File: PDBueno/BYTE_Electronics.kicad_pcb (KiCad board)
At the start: 2 copper layers, 99 x 42 mm, 3 parts, among them J9 Screw_Terminal_01x02, U1 LM2596S-3.3

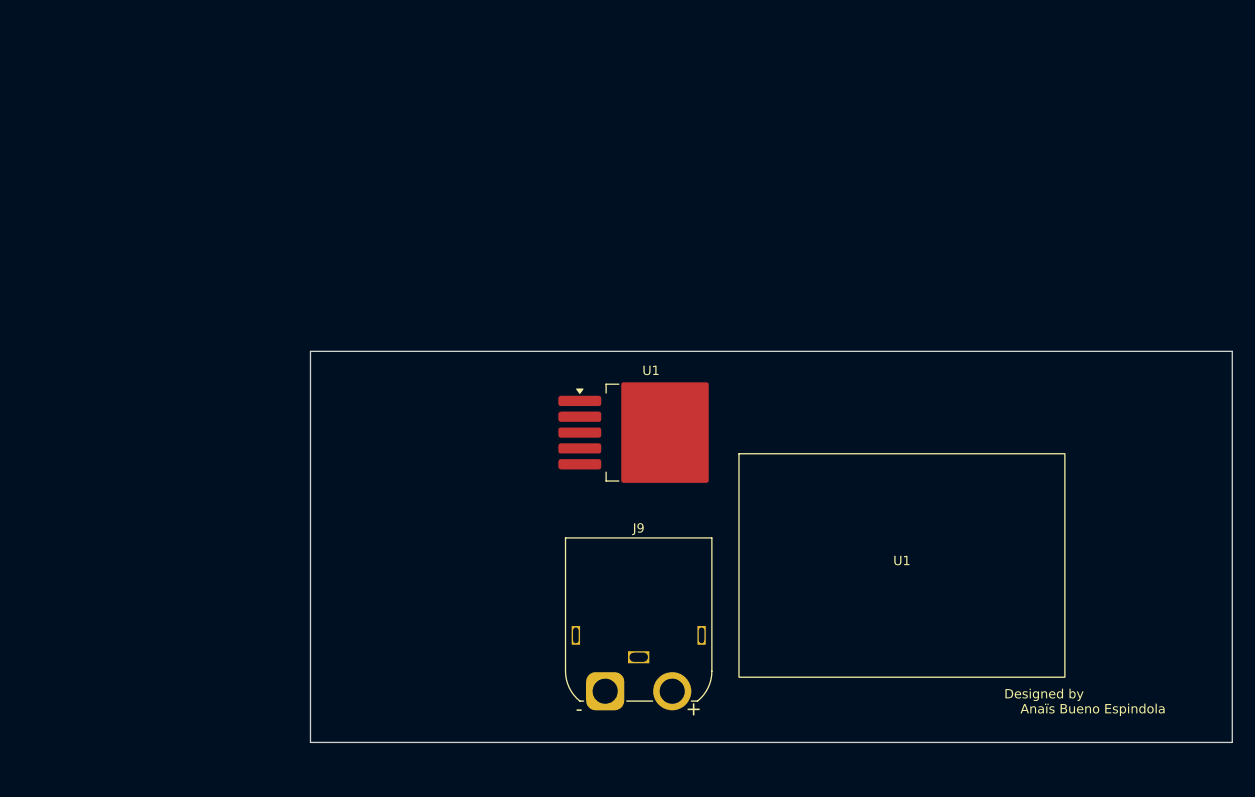
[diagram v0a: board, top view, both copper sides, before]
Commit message: PCB routing
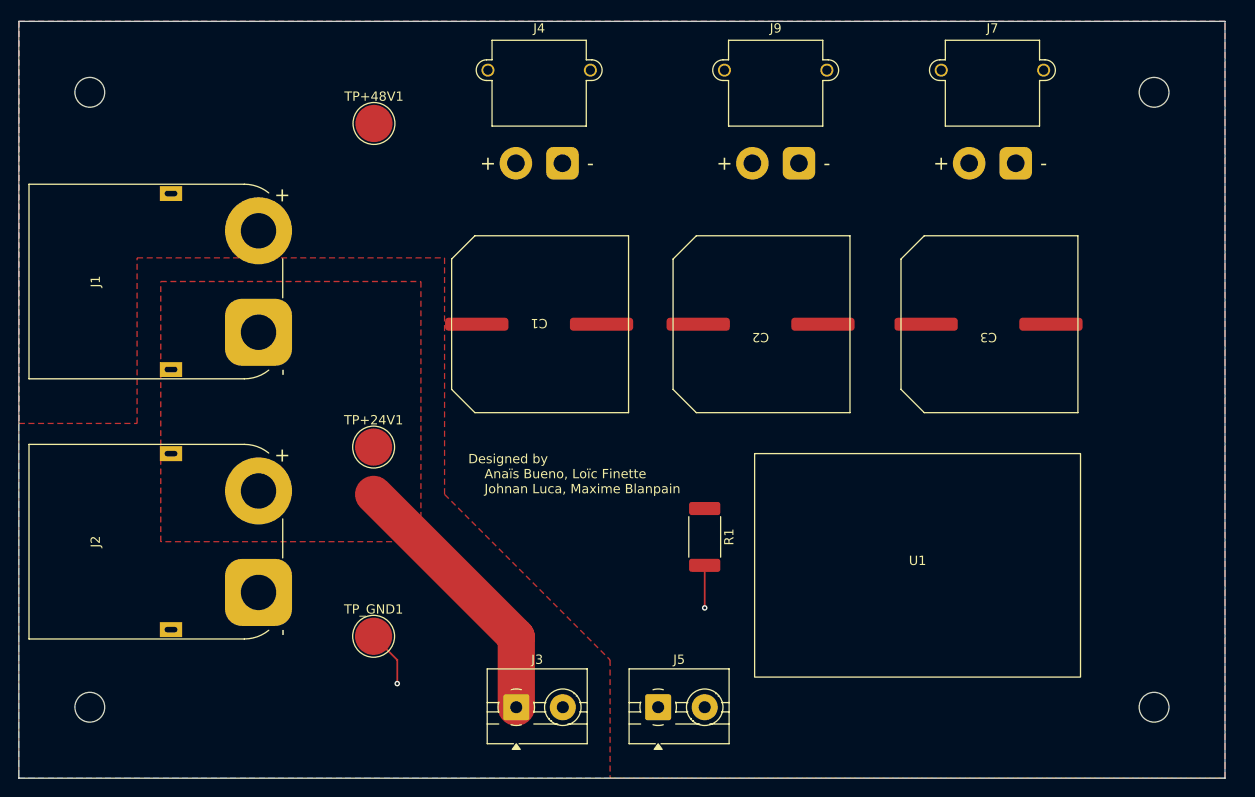
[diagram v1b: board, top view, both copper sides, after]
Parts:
- removed the U1 at (111.1, 79.7)
- added C1: 330uF, Footprint_PB_Byte:VZH331M2ATR-1816, F.Cu at (108.7, 58.6)
- added C2: 330uF, Footprint_PB_Byte:VZH331M2ATR-1816, F.Cu at (132.4, 58.6)
- added C3: 330uF, Footprint_PB_Byte:VZH331M2ATR-1816, F.Cu at (156.9, 58.6)
- added J1: Battery 2, Connector_AMASS:AMASS_XT90PW-M_1x02_P10.90mm_Horizontal, F.Cu at (68.9, 69.0)
- added J2: Battery 1, Connector_AMASS:AMASS_XT90PW-M_1x02_P10.90mm_Horizontal, F.Cu at (68.9, 96.9)
- added J3: Battery Buck 24V, TerminalBlock:TerminalBlock_MaiXu_MX126-5.0-02P_1x02_P5.00mm, F.Cu at (96.6, 109.2)
- added J4: Screw_Terminal_01x02, Connector_AMASS:AMASS_XT30PW-M_1x02_P2.50mm_Horizontal, F.Cu at (101.6, 50.8)
- added J5: Battery Buck 48V, TerminalBlock:TerminalBlock_MaiXu_MX126-5.0-02P_1x02_P5.00mm, F.Cu at (111.8, 109.2)
- added J7: Screw_Terminal_01x02, Connector_AMASS:AMASS_XT30PW-M_1x02_P2.50mm_Horizontal, F.Cu at (150.2, 50.8)
- added R1: 100kohms, Resistor_SMD:R_2512_6332Metric_Pad1.40x3.35mm_HandSolder, F.Cu at (116.8, 90.9)
- added REF**: MountingHole_3.2mm_M3_DIN965, MountingHole:MountingHole_3.2mm_M3_DIN965, F.Cu at (165.1, 43.2)
- added REF**: MountingHole_3.2mm_M3_DIN965, MountingHole:MountingHole_3.2mm_M3_DIN965, F.Cu at (165.1, 109.2)
- added REF**: MountingHole_3.2mm_M3_DIN965, MountingHole:MountingHole_3.2mm_M3_DIN965, F.Cu at (50.8, 43.2)
- added REF**: MountingHole_3.2mm_M3_DIN965, MountingHole:MountingHole_3.2mm_M3_DIN965, F.Cu at (50.8, 109.2)
- added TP+24V1: TestPoint, TestPoint:TestPoint_Pad_D4.0mm, F.Cu at (81.3, 81.3)
- added TP+48V1: TestPoint, TestPoint:TestPoint_Pad_D4.0mm, F.Cu at (81.3, 46.5)
- added TP_GND1: TestPoint, TestPoint:TestPoint_Pad_D4.0mm, F.Cu at (81.3, 101.6)
- J9: footprint Connector_AMASS:AMASS_XT60IPW-M_1x03_P7.20mm_Horizontal -> Connector_AMASS:AMASS_XT30PW-M_1x02_P2.50mm_Horizontal
- U1: value LM2596S-3.3 -> Buck Converter
- moved J9 60.4 mm to (127.0, 50.8)
- moved U1 1.68 mm to (139.7, 94.0)
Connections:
- J9 pad 1: unconnected-(J9-Pin_1-Pad1) -> /+48V
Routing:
- net /+24V: track 0.00 -> 32.0 mm
- net GND: track 0.00 -> 10.7 mm, vias 0 -> 2
- added copper zone on F.Cu, net /+24V
- added copper zone on F.Cu, net /+48V
- added copper zone on B.Cu, net GND
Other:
- board size 99 x 42 mm -> 129.5 x 81.3 mm
- board text added: "Designed by Anaïs Bueno, Loïc Finette Johnan Luca, Maxime Blanpain"
- board text removed: "Designed by Anaïs Bueno Espindola"
